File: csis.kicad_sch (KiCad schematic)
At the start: 11 parts, among them J1 Rain, J10 wind_sensor, J2 LORA, J3 PRESSURE, J4 Thermocoupler, J5 ADS, J6 I2C_Level_shifter, J7 GSM_module, J8 Barrel_Jack_MountingPin, J9 ADS, U2 RASPI PICO W

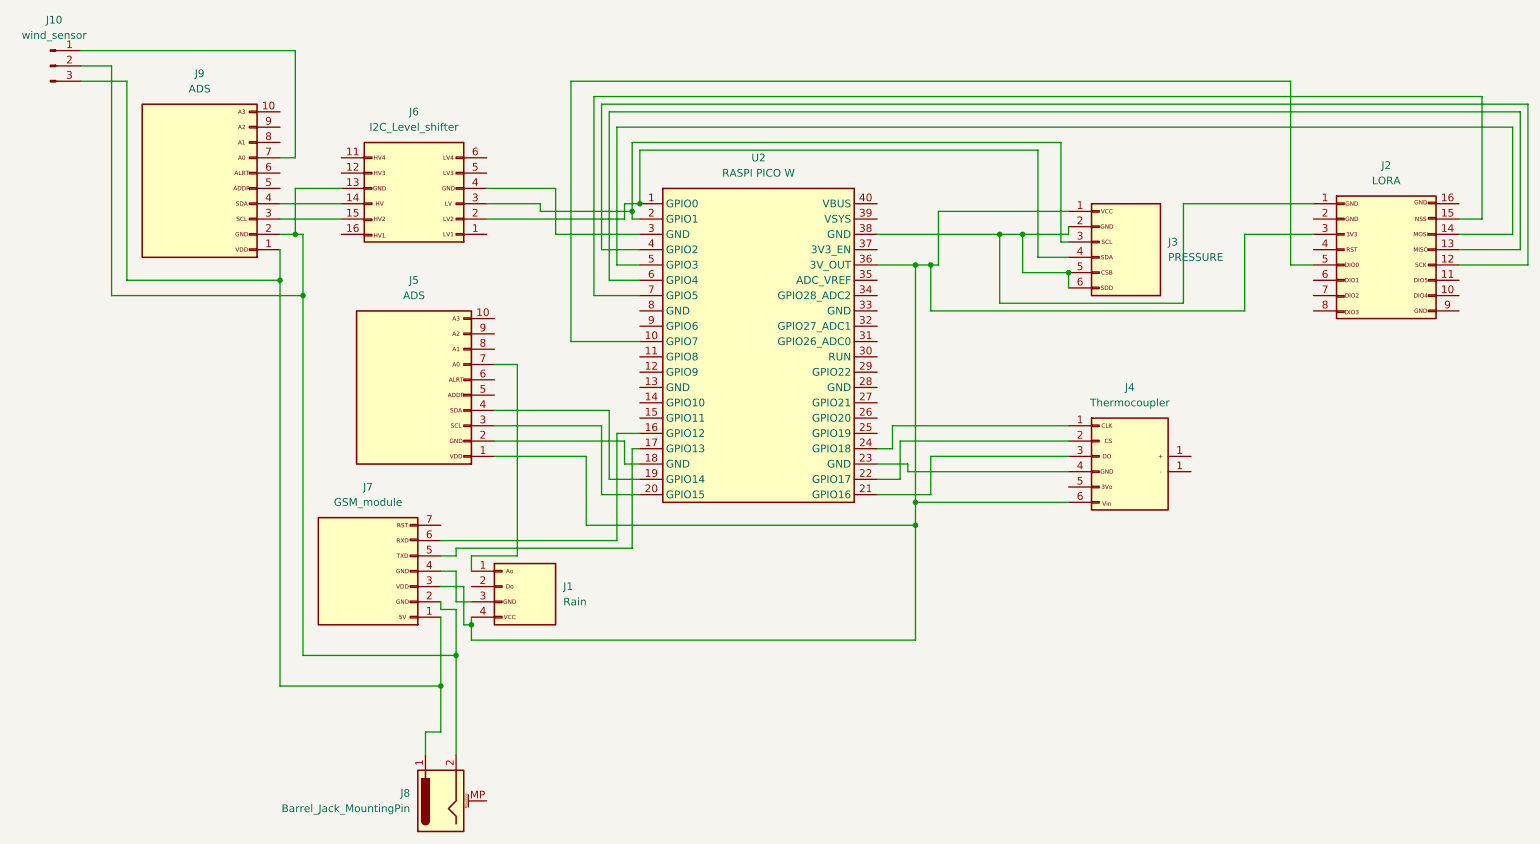
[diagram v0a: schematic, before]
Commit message: Add files via upload
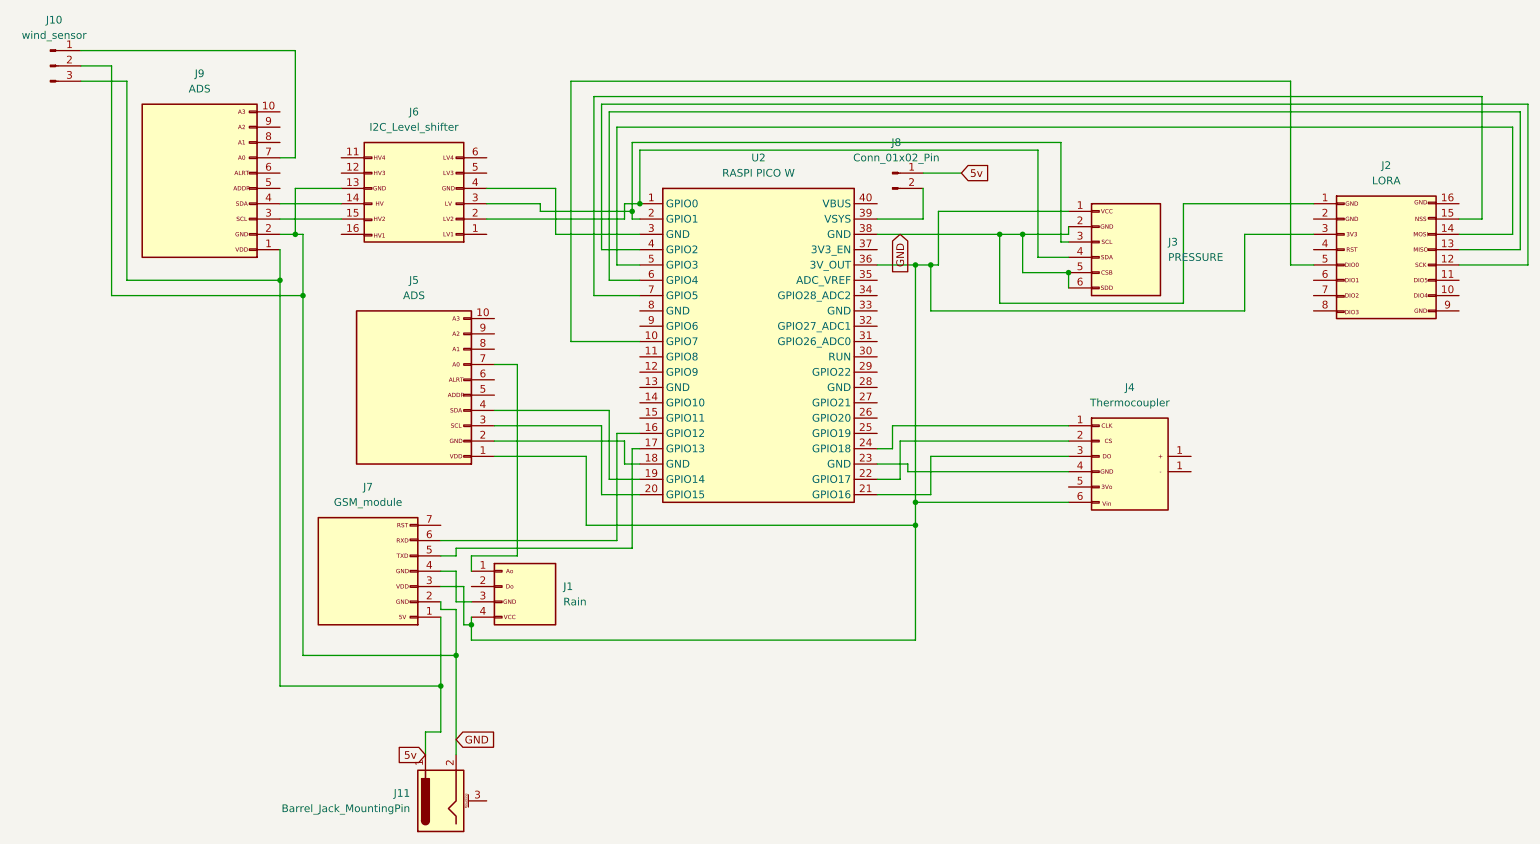
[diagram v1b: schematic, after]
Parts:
- removed J8: Barrel_Jack_MountingPin, Connector_BarrelJack:BarrelJack_Horizontal, symbol Connector:Barrel_Jack_MountingPin
- added J11: Barrel_Jack_MountingPin, Connector_BarrelJack:BarrelJack_Horizontal, symbol Connector:Barrel_Jack_MountingPin
- added J8: Conn_01x02_Pin, Connector_PinHeader_2.54mm:PinHeader_1x02_P2.54mm_Vertical, symbol Connector:Conn_01x02_Pin
- J6: footprint CSIS_LIB:BARO -> CSIS_LIB:i2c_level
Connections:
- net GND: now reaches J10.2 (Pin_2), J6.13 (Pin_5), J7.2 (Pin_2), J9.2 (Pin_2)
- net GND: now also J2.1 (Pin_1), J3.2 (Pin_2), J3.5 (Pin_5), J3.6 (SDD), U2.38 (GND), J11.2
- net 5v: now reaches J10.3 (Pin_3), J7.1 (Pin_1), J9.1 (Pin_1)
- net 5v: now also J11.1, J8.1 (Pin_1)
- net at J4.1 (Pin_1): now also U2.24 (GPIO18)
- net at U2.39 (VSYS): now also J8.2 (Pin_2)
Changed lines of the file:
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@@
+	(wire
+		(pts
+			(xy 167.64 64.77) (xy 173.99 64.77)
+		)
+		(stroke
+			(width 0)
+			(type default)
+		)
+	)
 	(wire
 		(pts
@@
 	(wire
 		(pts
+			(xy 167.64 67.31) (xy 167.64 72.39)
+		)
+		(stroke
+			(width 0)
+			(type default)
+		)
+	)
+	(wire
+		(pts
 			(xy 120.65 69.85) (xy 120.65 60.96)
 		)
@@
 	(wire
 		(pts
+			(xy 167.64 72.39) (xy 160.02 72.39)
+		)
+		(stroke
+			(width 0)
+			(type default)
+		)
+	)
+	(wire
+		(pts
 			(xy 191.77 74.93) (xy 191.77 73.66)
 		)
@@
 			(width 0)
 			(type default)
+		)
+	)
+	(global_label "GND"
+		(shape input)
+		(at 90.17 158.75 0)
+		(fields_autoplaced yes)
+		(effects
+			(font
+				(size 1.27 1.27)
+			)
+			(justify left)
+		)
+		(property "Intersheetrefs" "${INTERSHEET_REFS}"
+			(at 97.0257 158.75 0)
+			(effects
+				(font
+					(size 1.27 1.27)
+				)
+				(justify left)
+				(hide yes)
+			)
+		)
+	)
+	(global_label "GND"
+		(shape input)
+		(at 163.83 74.93 270)
+		(fields_autoplaced yes)
+		(effects
+			(font
+				(size 1.27 1.27)
+			)
+			(justify right)
+		)
+		(property "Intersheetrefs" "${INTERSHEET_REFS}"
+			(at 163.83 81.7857 90)
+			(effects
+				(font
+					(size 1.27 1.27)
+				)
+				(justify right)
+				(hide yes)
+			)
+		)
+	)
+	(global_label "5v"
+		(shape input)
+		(at 85.09 161.29 180)
+		(fields_autoplaced yes)
+		(effects
+			(font
+				(size 1.27 1.27)
+			)
+			(justify right)
+		)
+		(property "Intersheetrefs" "${INTERSHEET_REFS}"
+			(at 79.9277 161.29 0)
+			(effects
+				(font
+					(size 1.27 1.27)
+				)
+				(justify right)
+				(hide yes)
+			)
+		)
+	)
+	(global_label "5v"
+		(shape input)
+		(at 173.99 64.77 0)
+		(fields_autoplaced yes)
+		(effects
+			(font
+				(size 1.27 1.27)
+			)
+			(justify left)
+		)
+		(property "Intersheetrefs" "${INTERSHEET_REFS}"
+			(at 179.1523 64.77 0)
+			(effects
+				(font
+					(size 1.27 1.27)
+				)
+				(justify left)
+				(hide yes)
+			)
 		)
 	)
@@
 			)
 		)
-		(property "Footprint" "CSIS_LIB:BARO"
+		(property "Footprint" "CSIS_LIB:i2c_level"
 			(at 90.17 69.85 0)
 			(effects
@@
 	)
 	(symbol
+		(lib_name "Barrel_Jack_MountingPin_1")
+		(lib_id "Connector:Barrel_Jack_MountingPin")
+		(at 87.63 168.91 90)
+		(unit 1)
+		(exclude_from_sim no)
+		(in_bom yes)
+		(on_board yes)
+		(dnp no)
+		(fields_autoplaced yes)
+		(property "Reference" "J11"
+			(at 82.55 167.6399 90)
+			(effects
+				(font
+					(size 1.27 1.27)
+				)
+				(justify left)
+			)
+		)
+		(property "Value" "Barrel_Jack_MountingPin"
+			(at 82.55 170.1799 90)
+			(effects
+				(font
+					(size 1.27 1.27)
+				)
+				(justify left)
+			)
+		)
+		(property "Footprint" "Connector_BarrelJack:BarrelJack_Horizontal"
+			(at 88.646 167.64 0)
+			(effects
+				(font
+					(size 1.27 1.27)
+				)
+				(hide yes)
+			)
+		)
+		(property "Datasheet" "~"
+			(at 88.646 167.64 0)
+			(effects
+				(font
+					(size 1.27 1.27)
+				)
+				(hide yes)
+			)
+		)
+		(property "Description" "DC Barrel Jack with a mounting pin"
+			(at 87.63 168.91 0)
+			(effects
+				(font
+					(size 1.27 1.27)
+				)
+				(hide yes)
+			)
+		)
+		(pin "3"
+		)
+		(pin "1"
+		)
+		(pin "2"
+		)
+		(instances
+			(project ""
+				(path "/02eea2c5-5dd6-42fd-aeeb-0f452d907217"
+					(reference "J11")
+					(unit 1)
+				)
+			)
+		)
+	)
+	(symbol
 		(lib_name "Conn_01x06_2")
 		(lib_id "Connector_Generic:Conn_01x06")
@@
 	)
 	(symbol
-		(lib_id "Connector:Barrel_Jack_MountingPin")
-		(at 87.63 168.91 90)
+		(lib_id "Connector:Conn_01x02_Pin")
+		(at 162.56 64.77 0)
 		(unit 1)
 		(exclude_from_sim no)
@@
 		(fields_autoplaced yes)
 		(property "Reference" "J8"
-			(at 82.55 167.6399 90)
-			(effects
-				(font
-					(size 1.27 1.27)
-				)
-				(justify left)
-			)
-		)
-		(property "Value" "Barrel_Jack_MountingPin"
-			(at 82.55 170.1799 90)
-			(effects
-				(font
-					(size 1.27 1.27)
-				)
-				(justify left)
-			)
-		)
-		(property "Footprint" "Connector_BarrelJack:BarrelJack_Horizontal"
-			(at 88.646 167.64 0)
+			(at 163.195 59.69 0)
+			(effects
+				(font
+					(size 1.27 1.27)
+				)
+			)
+		)
+		(property "Value" "Conn_01x02_Pin"
+			(at 163.195 62.23 0)
+			(effects
+				(font
+					(size 1.27 1.27)
+				)
+			)
+		)
+		(property "Footprint" "Connector_PinHeader_2.54mm:PinHeader_1x02_P2.54mm_Vertical"
+			(at 162.56 64.77 0)
 			(effects
 				(font
@@
 		)
 		(property "Datasheet" "~"
-			(at 88.646 167.64 0)
-			(effects
-				(font
-					(size 1.27 1.27)
-				)
-				(hide yes)
-			)
-		)
-		(property "Description" "DC Barrel Jack with a mounting pin"
-			(at 87.63 168.91 0)
-			(effects
-				(font
-					(size 1.27 1.27)
-				)
-				(hide yes)
-			)
+			(at 162.56 64.77 0)
+			(effects
+				(font
+					(size 1.27 1.27)
+				)
+				(hide yes)
+			)
+		)
+		(property "Description" "Generic connector, single row, 01x02, script generated"
+			(at 162.56 64.77 0)
+			(effects
+				(font
+					(size 1.27 1.27)
+				)
+				(hide yes)
+			)
+		)
+		(pin "1"
 		)
 		(pin "2"
 		)
-		(pin "1"
-		)
-		(pin "MP"
-		)
 		(instances
